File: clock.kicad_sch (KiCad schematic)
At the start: 39 parts, among them SW1 Step, SW12 RESET, SW2 Clk Source, SW2 Run / Step, U1 LM555, U15 LM555, U2 LM555, U3 LM555, U4 74LS04, U5 74LS08, U6 74LS32, X1 ACO-xxxMHz

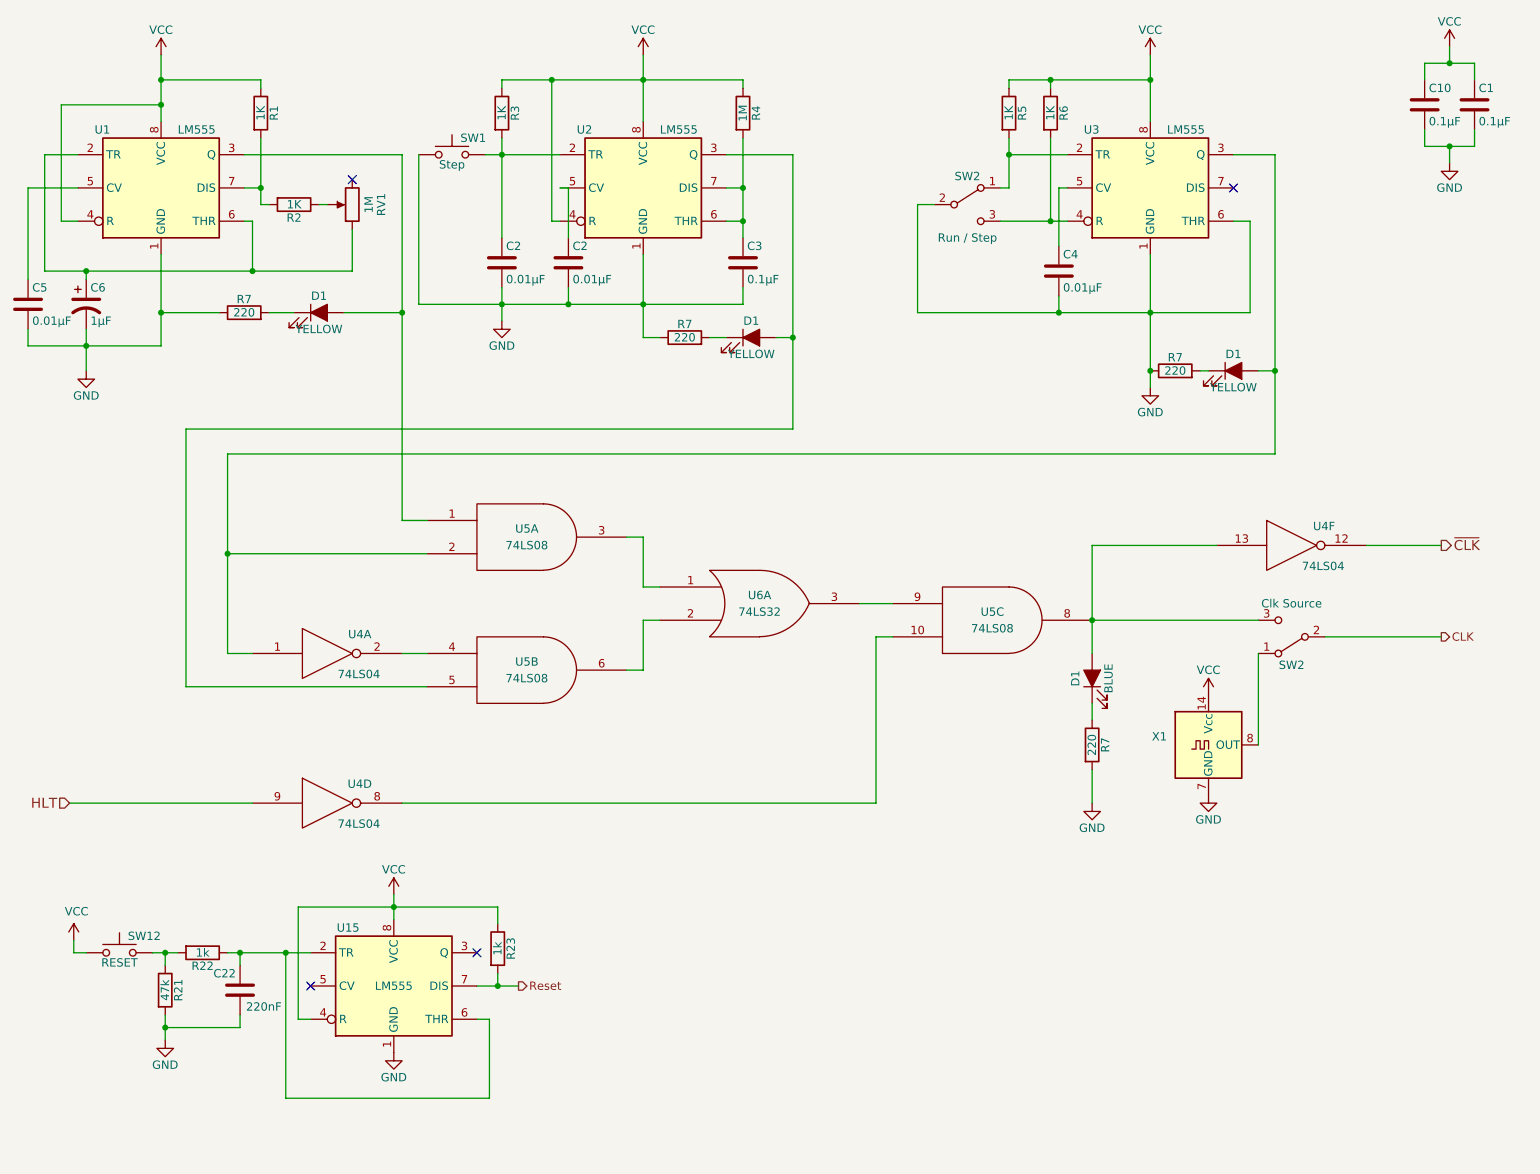
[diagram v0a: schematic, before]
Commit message: intermediate commit
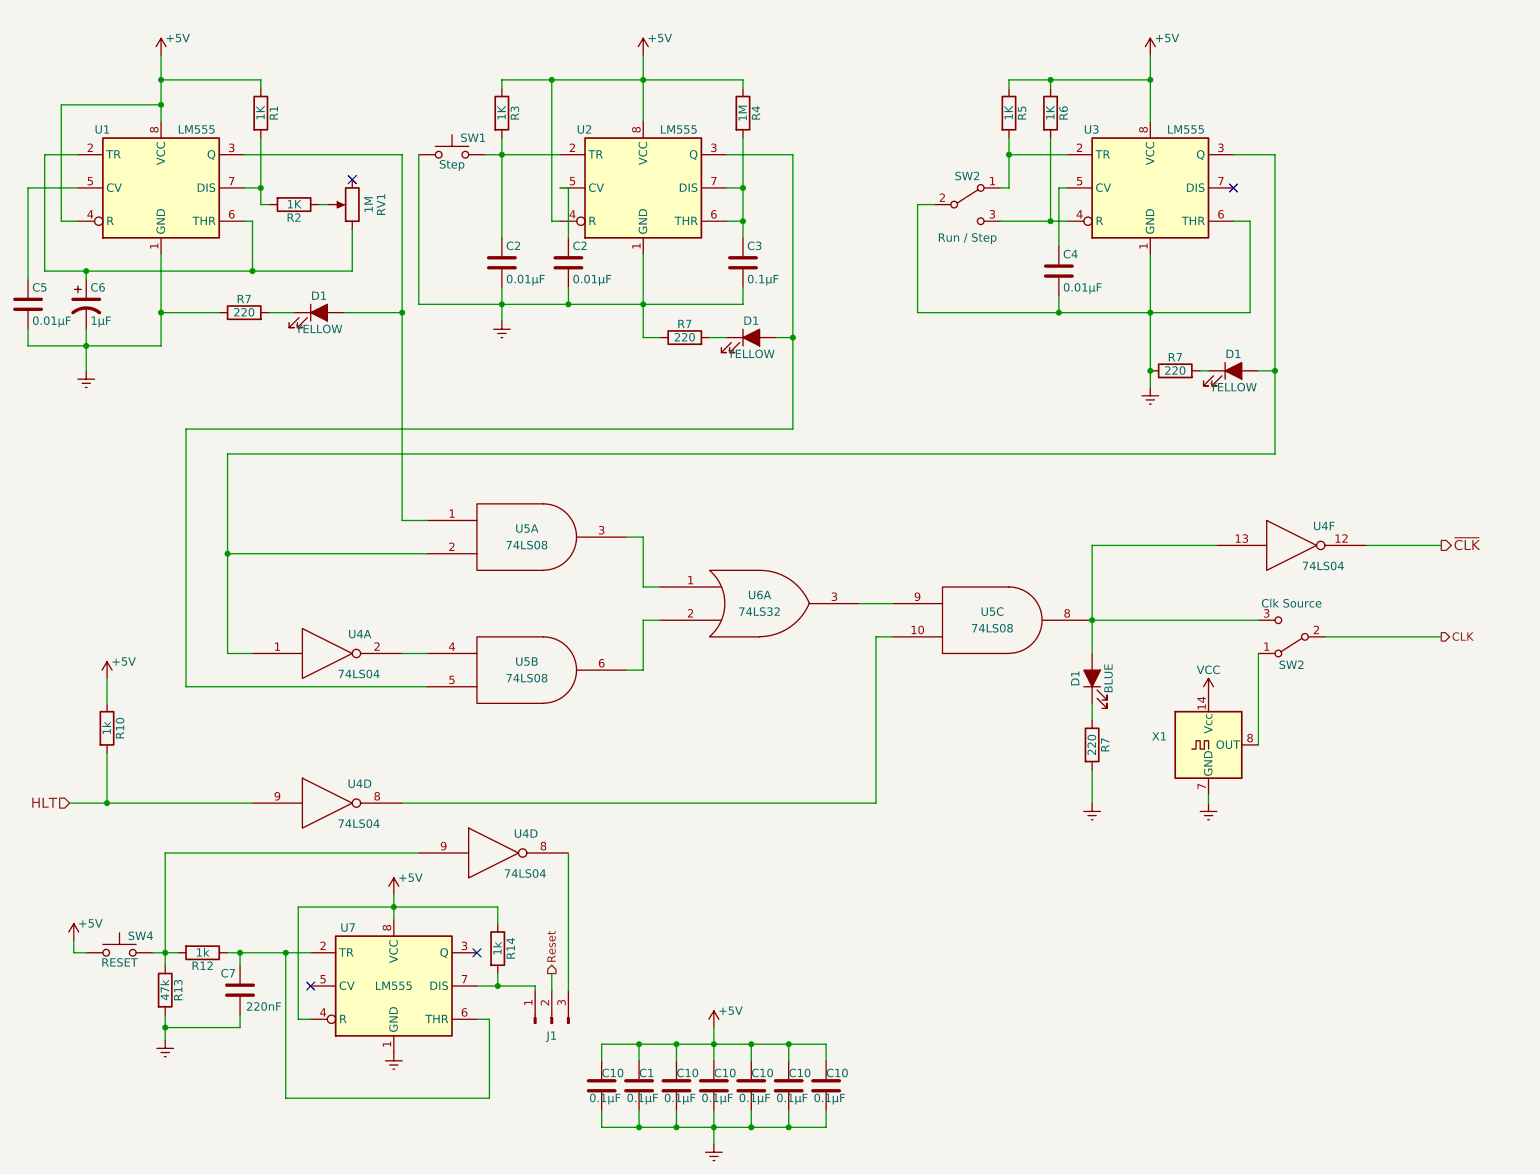
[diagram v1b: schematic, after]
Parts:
- added C10 (x5): 0.1µF, Capacitor_THT:C_Disc_D4.3mm_W1.9mm_P5.00mm, symbol Device:C
- added J1: Conn_01x03_Pin, Connector_PinSocket_1.27mm:PinSocket_1x03_P1.27mm_Vertical, symbol Connector:Conn_01x03_Pin
- added R10: 1k, Resistor_THT:R_Axial_DIN0207_L6.3mm_D2.5mm_P7.62mm_Horizontal, symbol Device:R
- added U4: 74LS04, Package_DIP:DIP-14_W7.62mm, symbol 8bit-computer-rescue:74LS04-8bit-computer-rescue
- renumbered C22 to C7, R22 to R12, R21 to R13, R23 to R14, SW12 to SW4, U15 to U7
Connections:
- net GND: now also U4.7 (GND); no longer C1.2, C10.2, C2.2, C2.2, C3.2, C4.2, C5.2, C6.2, C7.2, R13.2, R7.1, R7.1, R7.1, R7.2, SW1.1, SW2.2 (B), U1.1 (GND), U2.1 (GND), U3.1 (GND), U3.6 (THR), U7.1 (GND), X1.7 (GND)
- net HLT: now also R10.2
- net Reset: now also J1.2 (Pin_2); no longer R14.2, U7.7 (DIS)
- net VCC: now also U4.14 (VCC); no longer C1.1, C10.1, R1.1, R14.1, R3.1, R4.1, R5.1, R6.1, SW4.1, U1.4 (R), U1.8 (VCC), U2.4 (R), U2.8 (VCC), U3.8 (VCC), U7.4 (R), U7.8 (VCC)
- net at R12.2, R13.1, SW4.2: now also U4.9
- new net: J1.1 (Pin_1), R14.2, U7.7 (DIS)
- new net: J1.3 (Pin_3), U4.8
- new net +5V: C1.1, C10.1, C10.1, C10.1, C10.1, C10.1, C10.1, R1.1, R10.1, R14.1, R3.1, R4.1, R5.1, R6.1, SW4.1, U1.4 (R), U1.8 (VCC), U2.4 (R), U2.8 (VCC), U3.8 (VCC), U7.4 (R), U7.8 (VCC)
- new net Earth: C1.2, C10.2, C10.2, C10.2, C10.2, C10.2, C10.2, C2.2, C2.2, C3.2, C4.2, C5.2, C6.2, C7.2, R13.2, R7.1, R7.1, R7.1, R7.2, SW1.1, SW2.2 (B), U1.1 (GND), U2.1 (GND), U3.1 (GND), U3.6 (THR), U7.1 (GND), X1.7 (GND)
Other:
- moved on the sheet: C1, C10
